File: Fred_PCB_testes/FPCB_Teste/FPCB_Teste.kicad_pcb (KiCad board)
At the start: 2 copper layers, 17 parts, among them U1 SN65HVD230, U2 SN65HVD230, U3 MCP2515-xSO, Y1 Crystal

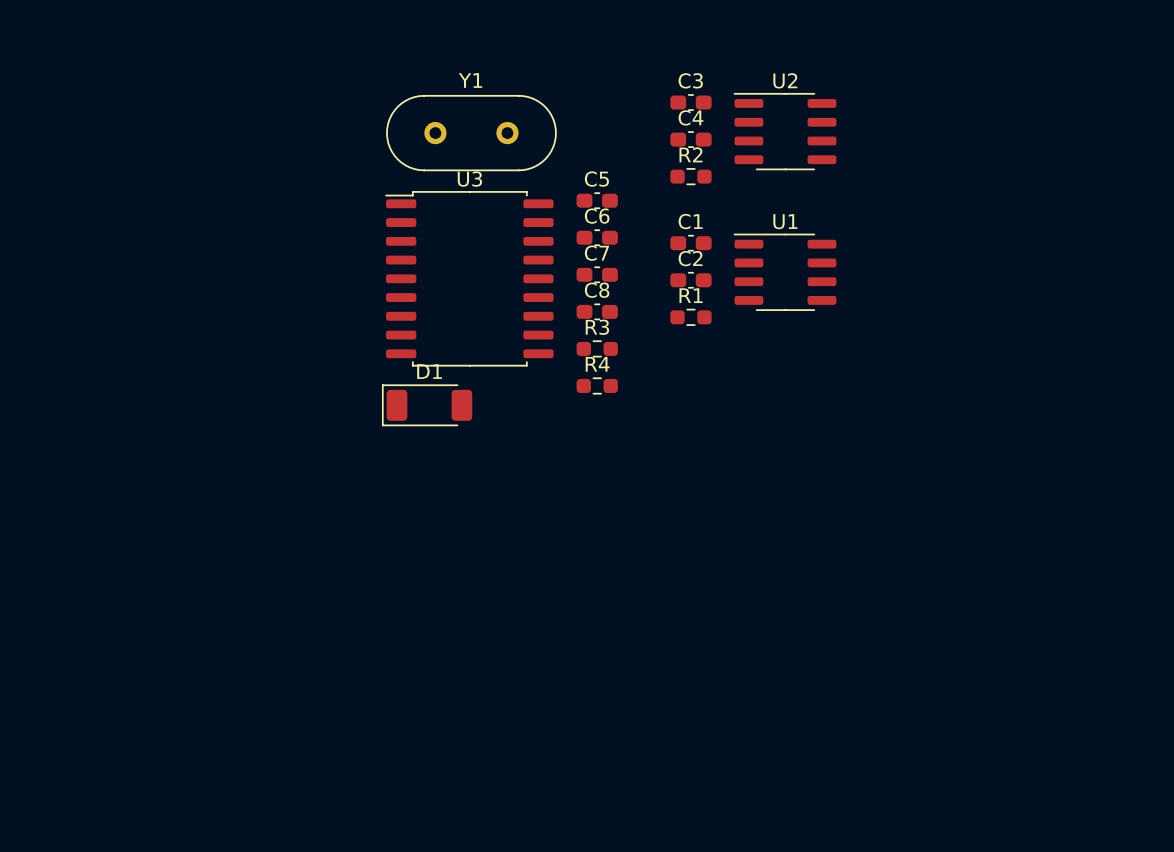
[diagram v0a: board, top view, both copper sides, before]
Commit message: Add files via upload
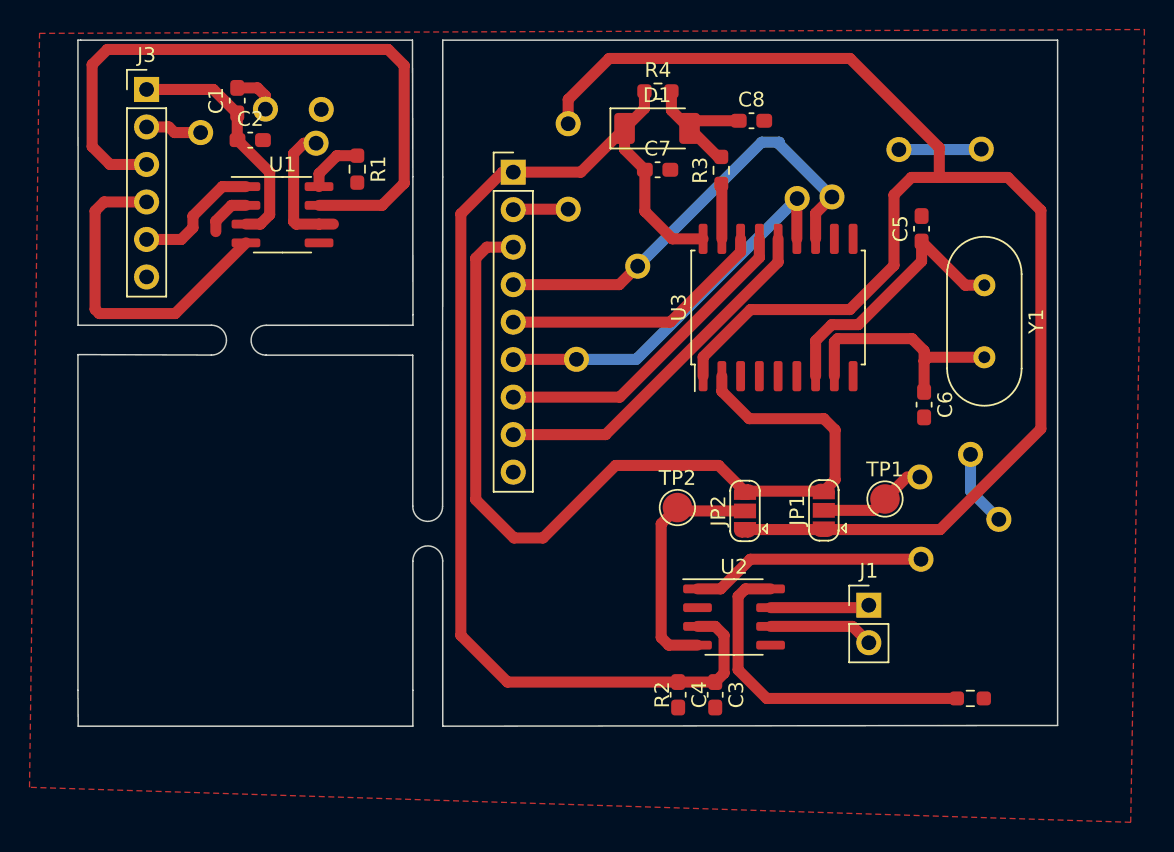
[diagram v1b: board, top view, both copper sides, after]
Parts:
- added ?: , , F.Cu at (170.9, 79.3)
- added ?: , , F.Cu at (136.3, 73.4)
- added ?: , , F.Cu at (176.8, 98.3)
- added ?: , , F.Cu at (128.1, 75.0)
- added ?: , , F.Cu at (176.9, 103.9)
- added ?: , , F.Cu at (157.7, 84.0)
- added ?: , , F.Cu at (180.2, 96.8)
- added ?: , , F.Cu at (135.9, 75.7)
- added ?: , , F.Cu at (168.5, 79.5)
- added ?: , , F.Cu at (153.5, 90.3)
- added ?: , , F.Cu at (175.4, 76.1)
- added ?: , , F.Cu at (182.2, 101.2)
- added ?: , , F.Cu at (132.5, 73.4)
- added ?: , , F.Cu at (153.0, 80.2)
- added ?: , , F.Cu at (181.0, 76.1)
- added ?: , , F.Cu at (153.0, 74.4)
- added J1: Conn_01x02, Connector_PinHeader_2.54mm:PinHeader_1x02_P2.54mm_Vertical, F.Cu at (173.4, 107.0)
- added J2: Conn_01x09, Connector_PinHeader_2.54mm:PinHeader_1x09_P2.54mm_Vertical, F.Cu at (149.3, 77.7)
- added J3: Conn_01x06, Connector_PinHeader_2.54mm:PinHeader_1x06_P2.54mm_Vertical, F.Cu at (124.4, 72.1)
- added JP1: SolderJumper_3_Open, Jumper:SolderJumper-3_P1.3mm_Open_RoundedPad1.0x1.5mm, F.Cu at (170.3, 100.6)
- added JP2: SolderJumper_3_Open, Jumper:SolderJumper-3_P1.3mm_Open_RoundedPad1.0x1.5mm, F.Cu at (165.0, 100.6)
- added TP1: TestPoint, TestPoint:TestPoint_Pad_D2.0mm, F.Cu at (174.4, 99.8)
- added TP2: TestPoint, TestPoint:TestPoint_Pad_D2.0mm, F.Cu at (160.4, 100.4)
- moved C3 40.2 mm to (162.9, 113.1), turned to -90 degrees
- moved R2 40.1 mm to (180.2, 113.3)
- moved Y1 38.6 mm to (181.2, 85.3), turned to -90 degrees
- moved C4 37.6 mm to (160.4, 113.1), turned to -90 degrees
- moved U1 34.3 mm to (133.6, 80.6)
- moved U2 33.1 mm to (164.2, 107.8)
- moved C1 32.2 mm to (130.6, 72.8), turned to 90 degrees
- moved C2 31.3 mm to (131.4, 75.5)
- moved C6 24.9 mm to (177.1, 93.4), turned to -90 degrees
- moved R1 24.7 mm to (138.7, 77.5), turned to -90 degrees
- moved D1 24.3 mm to (159.0, 74.7)
- moved C5 22.1 mm to (176.9, 81.5), turned to 90 degrees
- moved U3 21.0 mm to (167.2, 86.8), turned to 90 degrees
- moved R4 20.4 mm to (159.1, 72.2)
- moved C8 16.6 mm to (165.4, 74.2)
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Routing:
- net /MCP2515/TXCAN: track 0.00 -> 106.8 mm
- net 3,3v: track 0.00 -> 96.5 mm
- net /MCP2515/RXCAN: track 0.00 -> 60.9 mm
- net /SN65HVD230/CANH: track 0.00 -> 46.1 mm
- net /MCP2515/GPIO26: track 0.00 -> 30.6 mm
- net /MCP2515/GPIO11(SCLK): track 0.00 -> 26.5 mm
- net /MCP2515/GPIO10(MOSI): track 0.00 -> 24.4 mm
- net Net-(U2-Rs): track 0.00 -> 23.0 mm
- net /SN65HVD230/R: track 0.00 -> 22.7 mm
- net /SN65HVD231_RASP/D: track 0.00 -> 22.6 mm
- net /MCP2515/GPIO9(MISO): track 0.00 -> 21.9 mm
- net Net-(U3-OSC2): track 0.00 -> 18.6 mm
- net /MCP2515/GPIO22: track 0.00 -> 18.3 mm
- net GND: track 0.00 -> 17.0 mm
- net /SN65HVD231_RASP/R: track 0.00 -> 16.6 mm
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- added copper zone on F.Cu, net GND
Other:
- board outline added: 66.4 x 46.5 mm
